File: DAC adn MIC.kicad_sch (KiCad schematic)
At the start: 28 parts, among them J401 AudioJack2_Ground, J402 Conn_01x04_Pin, U401 CS43L22-CNZ, U402 IMP34DT05TR

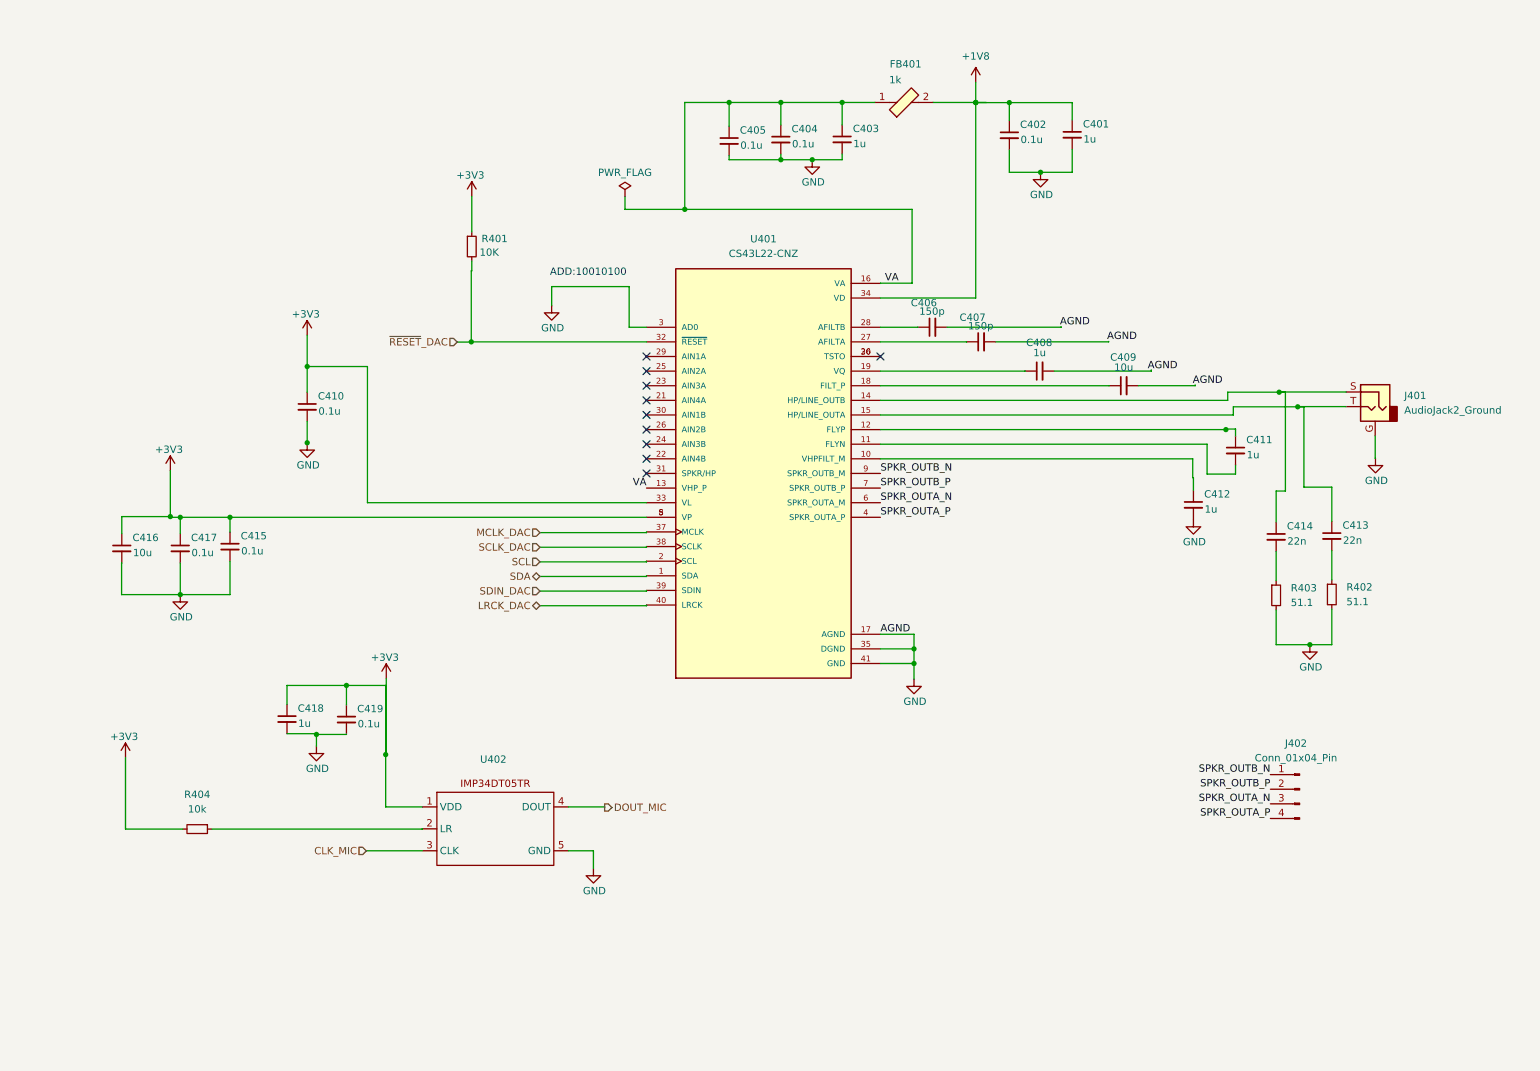
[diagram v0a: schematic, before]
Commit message: schematic pages are reviewed
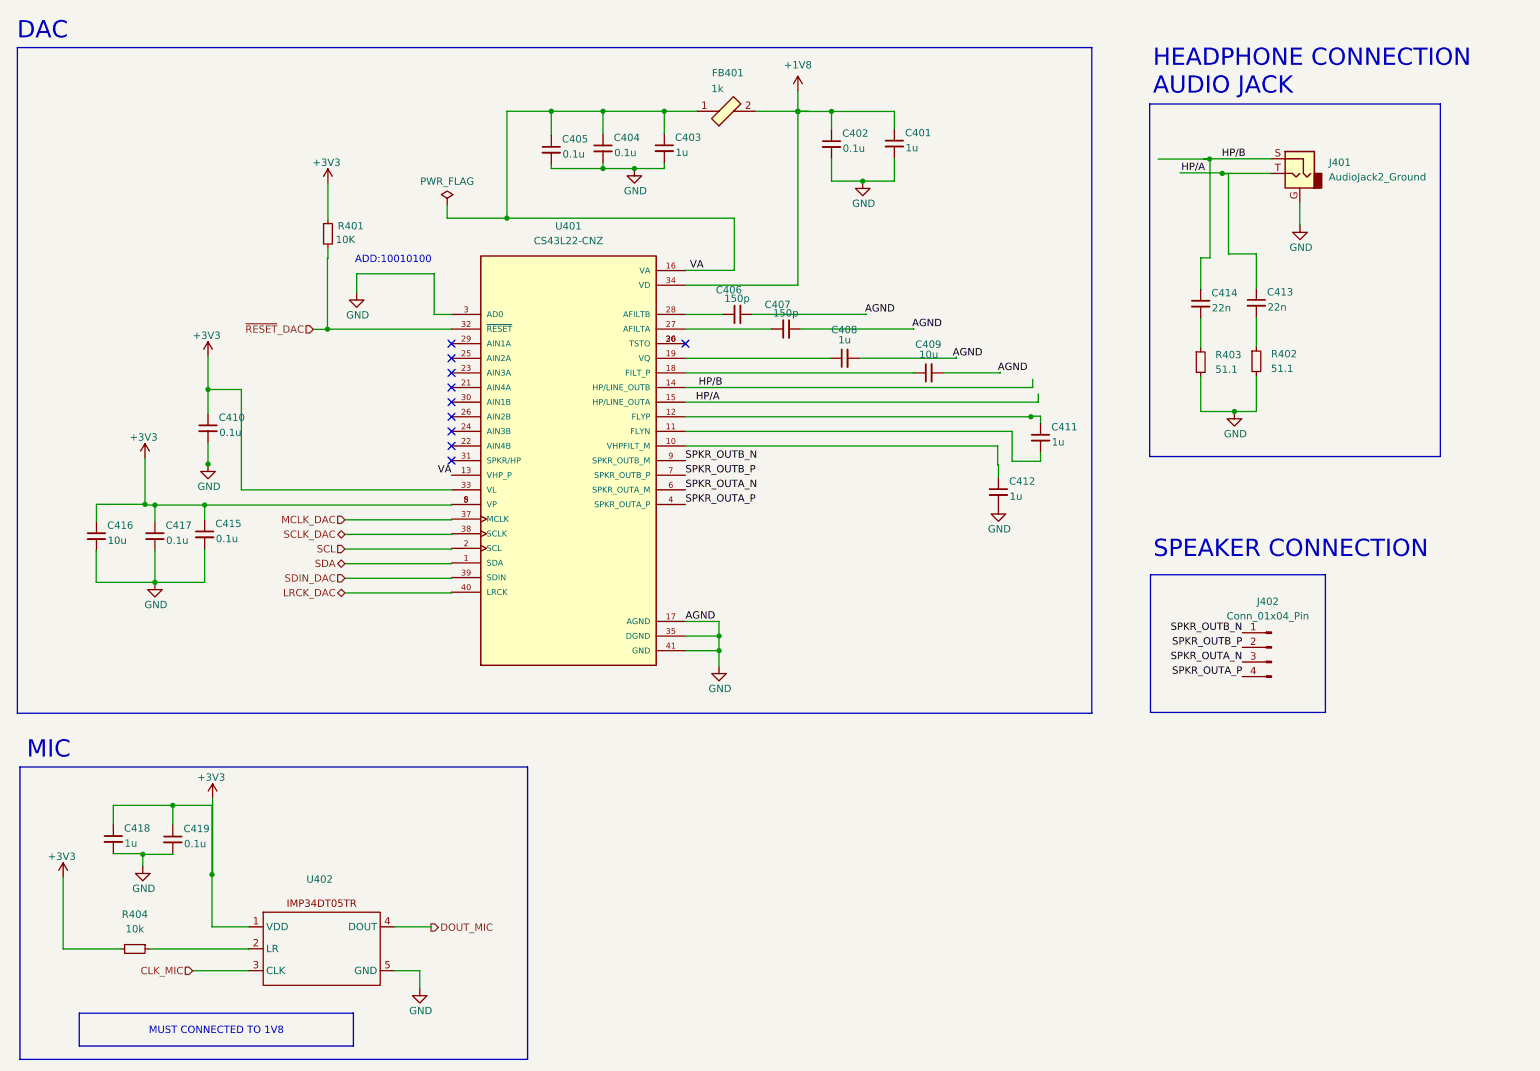
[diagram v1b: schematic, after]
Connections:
- net HP/B: now reaches C414.1, J401.S, U401.14 (HP/LINE_OUTB)
- net HP/A: now reaches C413.1, J401.T, U401.15 (HP/LINE_OUTA)
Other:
- note added: "DAC"
- note added: "HEADPHONE CONNECTION AUDIO JACK"
- note added: "MIC"
- note added: "SPEAKER CONNECTION"
- moved on the sheet: C401, C402, C403, C404, C405, C406, C407, C408, C409, C410, C411, C412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
